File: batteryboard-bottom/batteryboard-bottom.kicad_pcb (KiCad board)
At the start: 2 copper layers, 46.8 x 46.8 mm, 7 parts, among them J1 SFC-110-T2-F-D-A, J2 FTS-107-01-L-DV-A

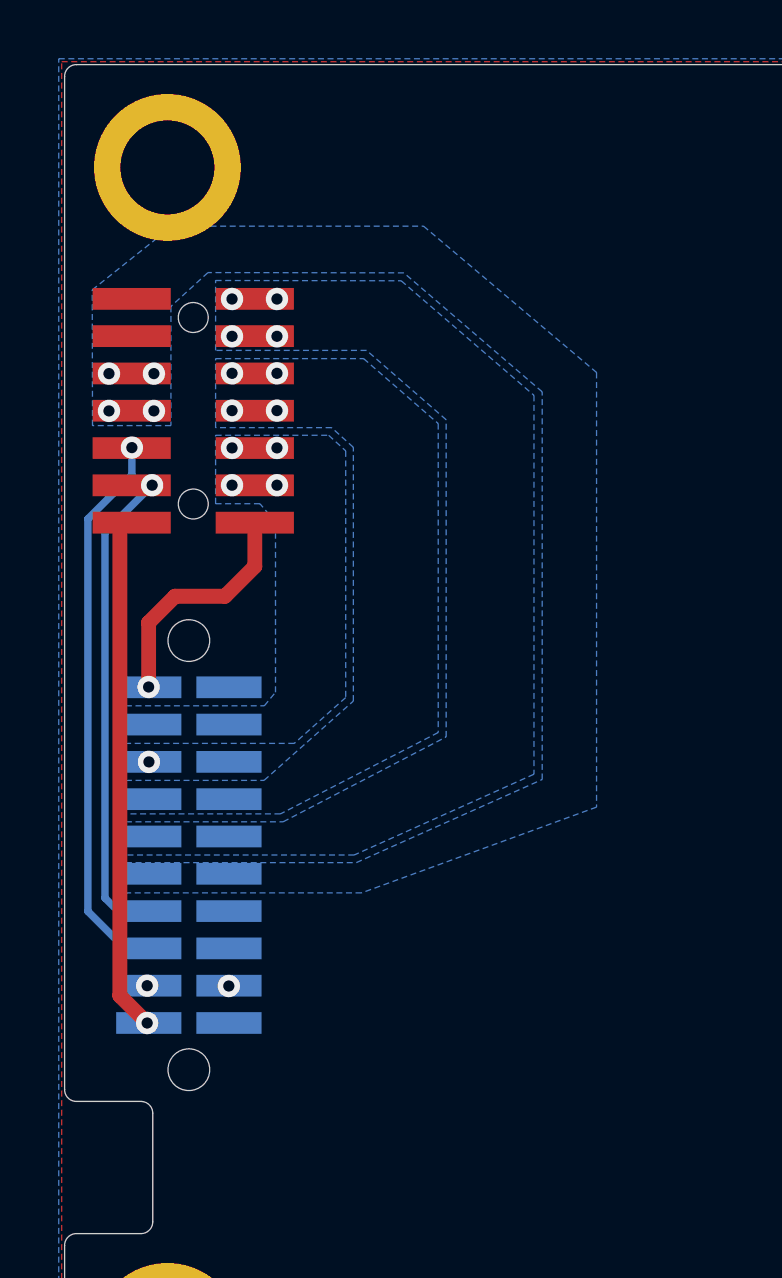
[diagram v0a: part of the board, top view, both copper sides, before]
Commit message: Minor updates and exported STEP / BOM
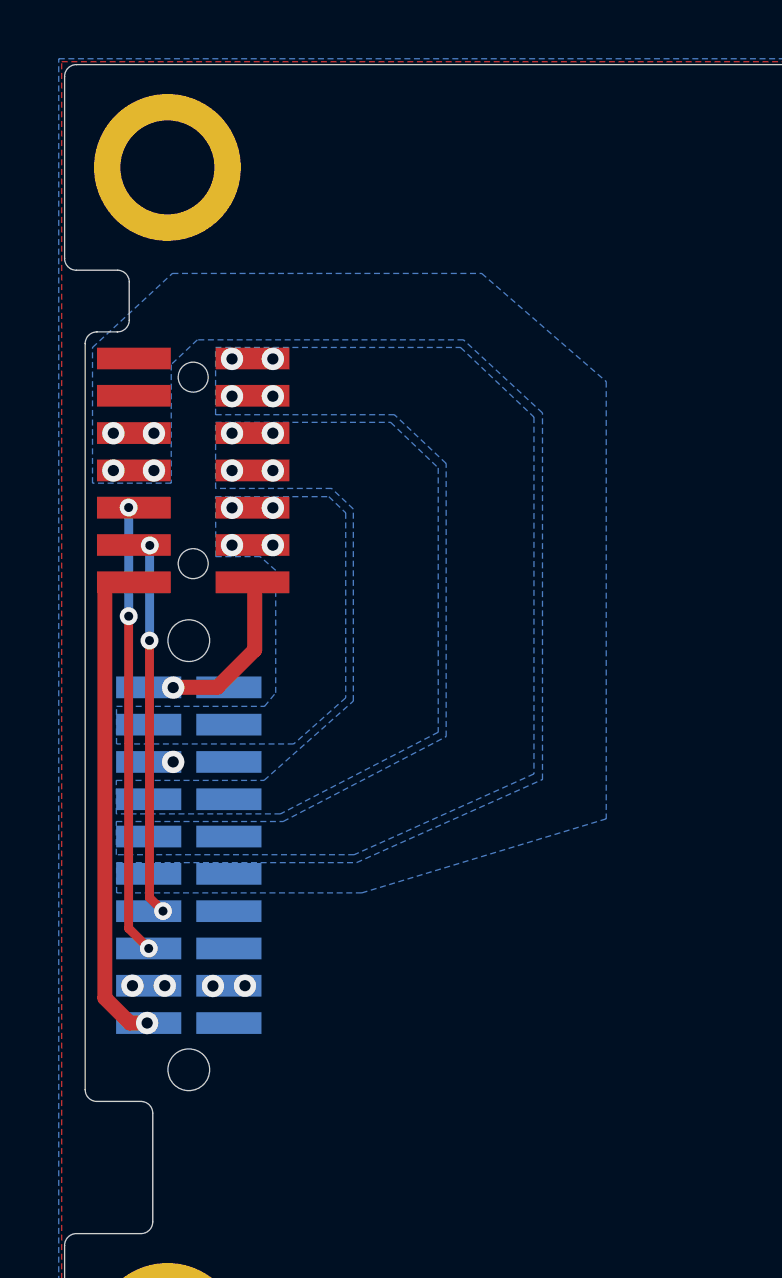
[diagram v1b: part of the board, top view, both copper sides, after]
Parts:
- moved J2 2.03 mm to (133.7, 92.1)
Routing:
- net SDA1: track 16.4 -> 12.6 mm, vias 1 -> 3
- net SCL1: track 18.2 -> 15.3 mm, vias 1 -> 3
- net COIL5_N: track 8.09 -> 5.61 mm
- net GND: vias 3 -> 5
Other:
- outline, holes or cut-outs redrawn
- board text added: "06-NOV-22"
- board text removed: "09-OCT-22"
